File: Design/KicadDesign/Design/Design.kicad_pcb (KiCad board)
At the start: 2 copper layers, 170.7 x 101 mm, 19 parts, among them J1 Speaker, J2 SourceSupply, J3 Jack 3.5 mm, J4 Conn_01x20_Socket, J5 Conn_01x20_Socket, Q1 IRLZ44N, Q2 IRLZ44N, U1 IR2110

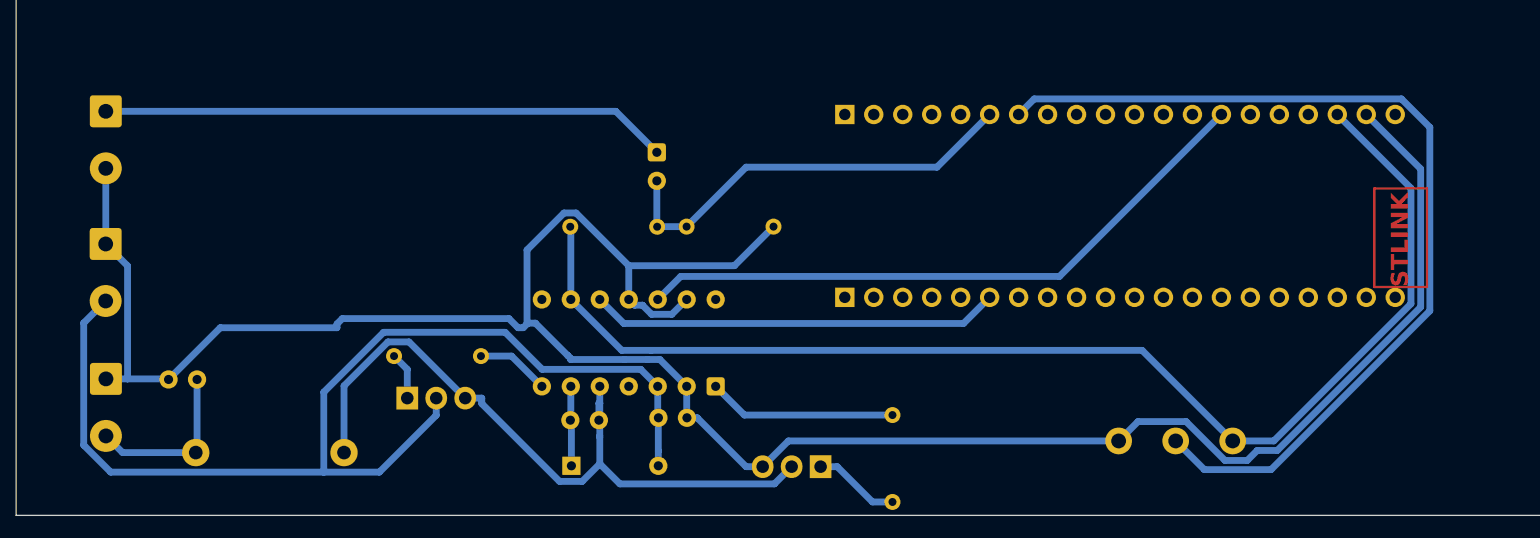
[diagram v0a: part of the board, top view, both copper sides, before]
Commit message: Minor fixes on traces
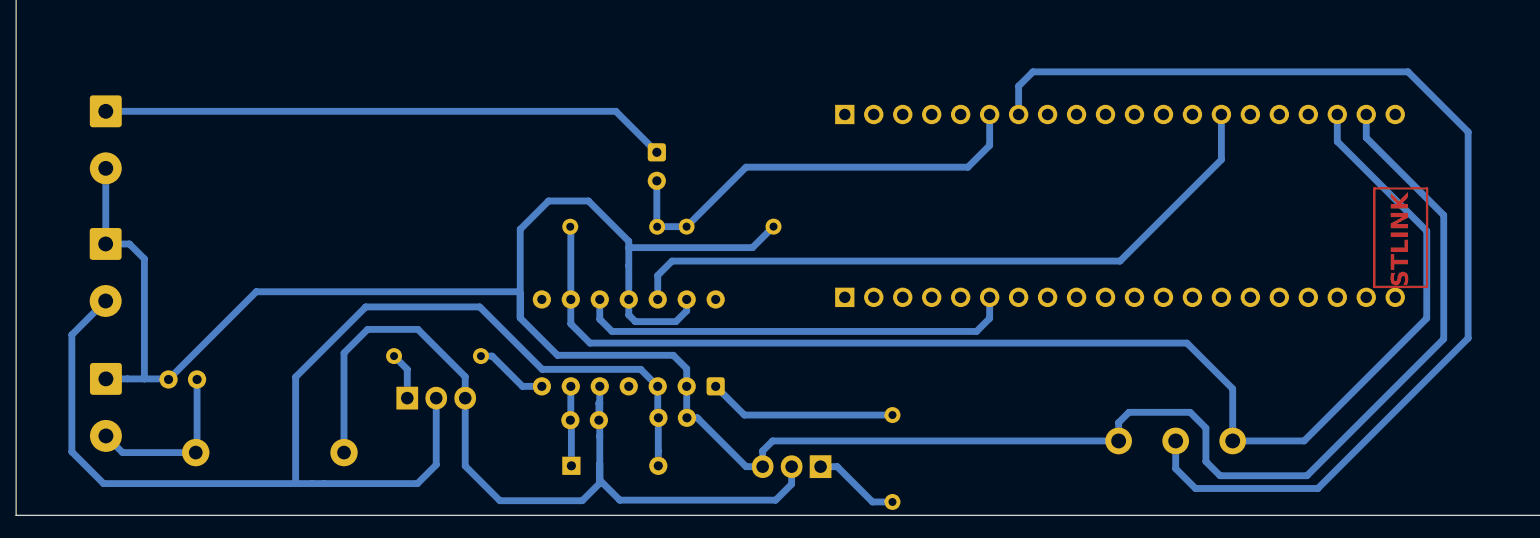
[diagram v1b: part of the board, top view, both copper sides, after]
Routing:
- net GND: track 213.7 -> 233.3 mm
- net A1 ADC2: track 82.8 -> 96.9 mm
- net Net-(Q1-S): track 62.4 -> 74.6 mm
- net 12V: track 96.3 -> 107.6 mm
- net 3.3V: track 109.4 -> 116.1 mm
- net B0 PWM_N: track 56.1 -> 59.7 mm
- net A9 PWM: track 36.0 -> 38.7 mm
- net A0 ADC1: track 37.3 -> 38.9 mm

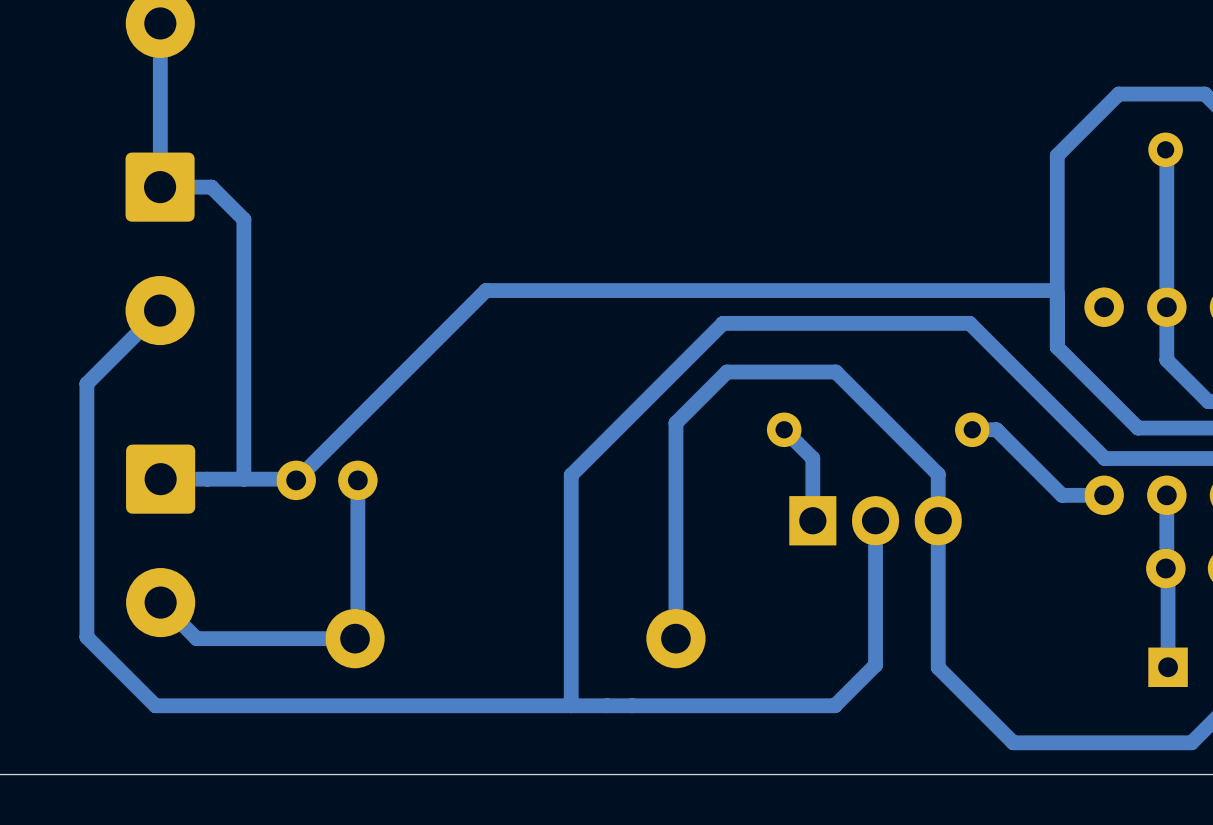
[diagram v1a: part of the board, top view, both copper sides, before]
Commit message: Minor fixes on traces
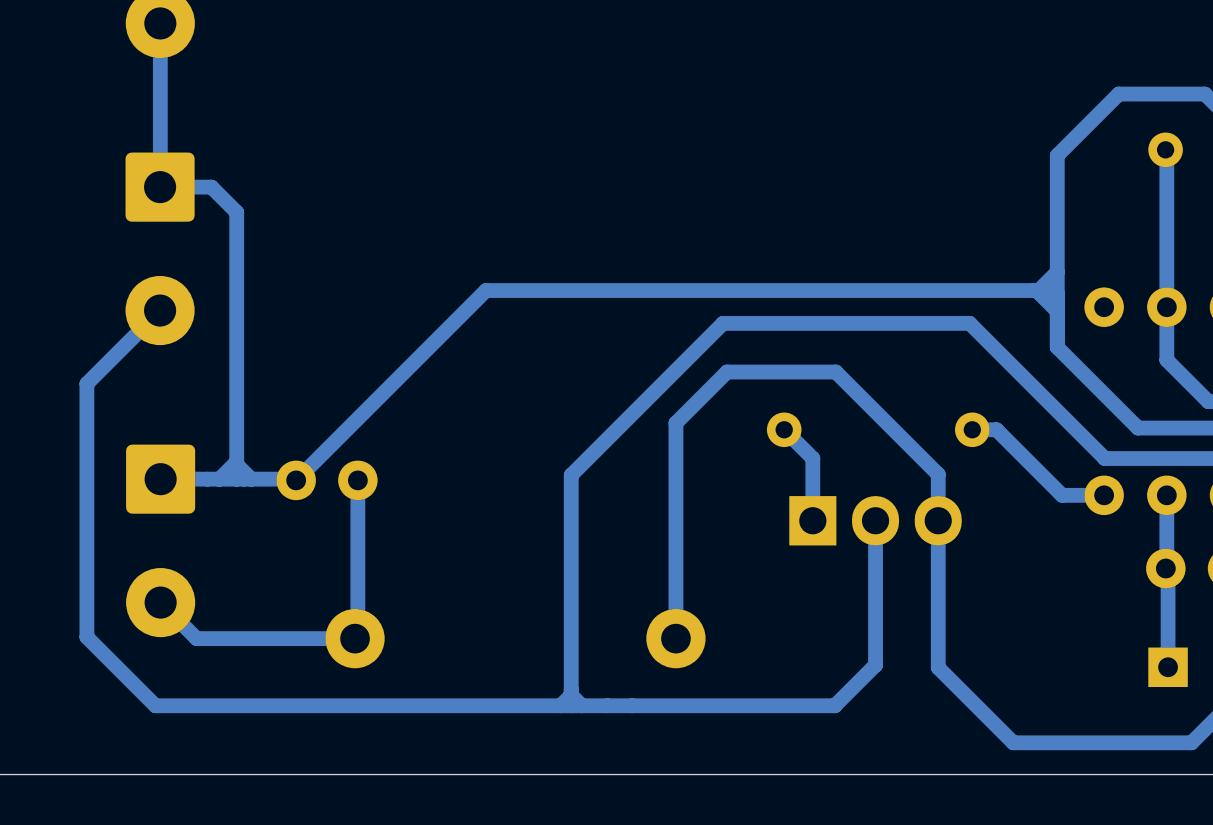
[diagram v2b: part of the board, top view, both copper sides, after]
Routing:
- net GND: track 233.3 -> 237.5 mm
- net 12V: track 107.6 -> 109.0 mm
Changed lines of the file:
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@@
+	)
+	(segment
+		(start 96.82 100.99)
+		(end 96.82 102.45)
+		(width 0.6)
+		(layer "B.Cu")
+		(net 1)
 	)
 	(segment
@@
 	)
 	(segment
+		(start 96.82 99.4)
+		(end 96.82 94.68)
+		(width 0.6)
+		(layer "B.Cu")
+		(net 1)
+	)
+	(segment
 		(start 156.94 115.04)
 		(end 158.18 116.28)
@@
 	)
 	(segment
+		(start 63.58 107.79)
+		(end 63.87 107.79)
+		(width 0.6)
+		(layer "B.Cu")
+		(net 1)
+	)
+	(segment
 		(start 112.3383 111.2)
 		(end 111.4375 111.2)
@@
 	)
 	(segment
+		(start 63.58 107.2)
+		(end 64.17 107.79)
+		(width 0.6)
+		(layer "B.Cu")
+		(net 1)
+	)
+	(segment
 		(start 149.2875 113.23)
 		(end 149.2875 111.6225)
@@
 	)
 	(segment
+		(start 96.07 100.24)
+		(end 96.82 100.99)
+		(width 0.6)
+		(layer "B.Cu")
+		(net 1)
+	)
+	(segment
+		(start 64.17 107.79)
+		(end 65.9375 107.79)
+		(width 0.6)
+		(layer "B.Cu")
+		(net 1)
+	)
+	(segment
 		(start 111.4375 111.2)
 		(end 111.4175 111.18)
@@
 	)
 	(segment
+		(start 63.58 107.09)
+		(end 63.58 107.79)
+		(width 0.6)
+		(layer "B.Cu")
+		(net 1)
+	)
+	(segment
 		(start 96.82 94.68)
 		(end 99.31 92.19)
@@
 	)
 	(segment
+		(start 95.9 100.15)
+		(end 96.07 100.15)
+		(width 0.6)
+		(layer "B.Cu")
+		(net 1)
+	)
+	(segment
+		(start 96.07 100.15)
+		(end 96.07 100.24)
+		(width 0.6)
+		(layer "B.Cu")
+		(net 1)
+	)
+	(segment
 		(start 100.09 105.72)
 		(end 96.82 102.45)
@@
 	)
 	(segment
+		(start 95.9 100.15)
+		(end 96.69 100.15)
+		(width 0.6)
+		(layer "B.Cu")
+		(net 1)
+	)
+	(segment
 		(start 99.31 92.19)
 		(end 102.8 92.19)
@@
 	)
 	(segment
+		(start 63.58 96.98)
+		(end 63.58 107.09)
+		(width 0.6)
+		(layer "B.Cu")
+		(net 1)
+	)
+	(segment
 		(start 60.475 95.96)
 		(end 62.56 95.96)
@@
 	)
 	(segment
+		(start 96.07 100.15)
+		(end 96.82 99.4)
+		(width 0.6)
+		(layer "B.Cu")
+		(net 1)
+	)
+	(segment
 		(start 96.82 100.28)
-		(end 96.82 102.45)
+		(end 96.82 100.99)
 		(width 0.6)
 		(layer "B.Cu")
@@
 	(segment
 		(start 62.3936 107.79)
-		(end 63.87 107.79)
+		(end 62.88 107.79)
 		(width 0.6)
 		(layer "B.Cu")
@@
 	(segment
 		(start 73.6775 100.15)
-		(end 96.69 100.15)
+		(end 95.9 100.15)
+		(width 0.6)
+		(layer "B.Cu")
+		(net 1)
+	)
+	(segment
+		(start 62.88 107.79)
+		(end 63.58 107.09)
 		(width 0.6)
 		(layer "B.Cu")
@@
 	)
 	(segment
-		(start 63.87 97.27)
-		(end 63.87 107.79)
+		(start 62.56 95.96)
+		(end 63.58 96.98)
 		(width 0.6)
 		(layer "B.Cu")
@@
 	)
 	(segment
+		(start 62.88 107.79)
+		(end 63.58 107.79)
+		(width 0.6)
+		(layer "B.Cu")
+		(net 1)
+	)
+	(segment
 		(start 118.0775 115.485)
 		(end 116.6233 115.485)
@@
 	(segment
 		(start 63.87 107.79)
-		(end 65.9375 107.79)
+		(end 64.17 107.79)
 		(width 0.6)
 		(layer "B.Cu")
@@
 	(segment
 		(start 96.82 102.45)
-		(end 96.82 94.68)
-		(width 0.6)
-		(layer "B.Cu")
-		(net 1)
-	)
-	(segment
-		(start 62.56 95.96)
-		(end 63.87 97.27)
+		(end 96.82 99.4)
 		(width 0.6)
 		(layer "B.Cu")
@@
 	)
 	(segment
+		(start 63.58 107.09)
+		(end 63.58 107.2)
+		(width 0.6)
+		(layer "B.Cu")
+		(net 1)
+	)
+	(segment
 		(start 158.18 116.28)
 		(end 165.8 116.28)
@@
 	(segment
 		(start 77.13 107.63)
-		(end 77.13 116.97)
+		(end 77.13 116.31)
 		(width 0.6)
 		(layer "B.Cu")
@@
 	)
 	(segment
+		(start 77.13 116.31)
+		(end 77.13 116.54)
+		(width 0.6)
+		(layer "B.Cu")
+		(net 3)
+	)
+	(segment
+		(start 60.29 116.97)
+		(end 76.7 116.97)
+		(width 0.6)
+		(layer "B.Cu")
+		(net 3)
+	)
+	(segment
+		(start 77.13 116.31)
+		(end 77.13 116.97)
+		(width 0.6)
+		(layer "B.Cu")
+		(net 3)
+	)
+	(segment
+		(start 77.13 116.54)
+		(end 76.7 116.97)
+		(width 0.6)
+		(layer "B.Cu")
+		(net 3)
+	)
+	(segment
 		(start 108.8775 111.15)
 		(end 108.8775 108.445)
@@
 	)
 	(segment
+		(start 77.13 116.54)
+		(end 77.56 116.97)
+		(width 0.6)
+		(layer "B.Cu")
+		(net 3)
+	)
+	(segment
 		(start 79.6 116.97)
 		(end 78.5941 116.97)
@@
 	)
 	(segment
-		(start 60.29 116.97)
+		(start 76.7 116.97)
 		(end 77.13 116.97)
+		(width 0.6)
+		(layer "B.Cu")
+		(net 3)
+	)
+	(segment
+		(start 77.13 116.97)
+		(end 77.56 116.97)
 		(width 0.6)
 		(layer "B.Cu")
@@
 	)
 	(segment
-		(start 77.13 116.97)
+		(start 77.56 116.97)
 		(end 78.5941 116.97)
 		(width 0.6)
